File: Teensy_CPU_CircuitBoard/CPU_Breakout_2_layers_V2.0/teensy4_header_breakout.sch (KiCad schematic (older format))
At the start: 0 parts

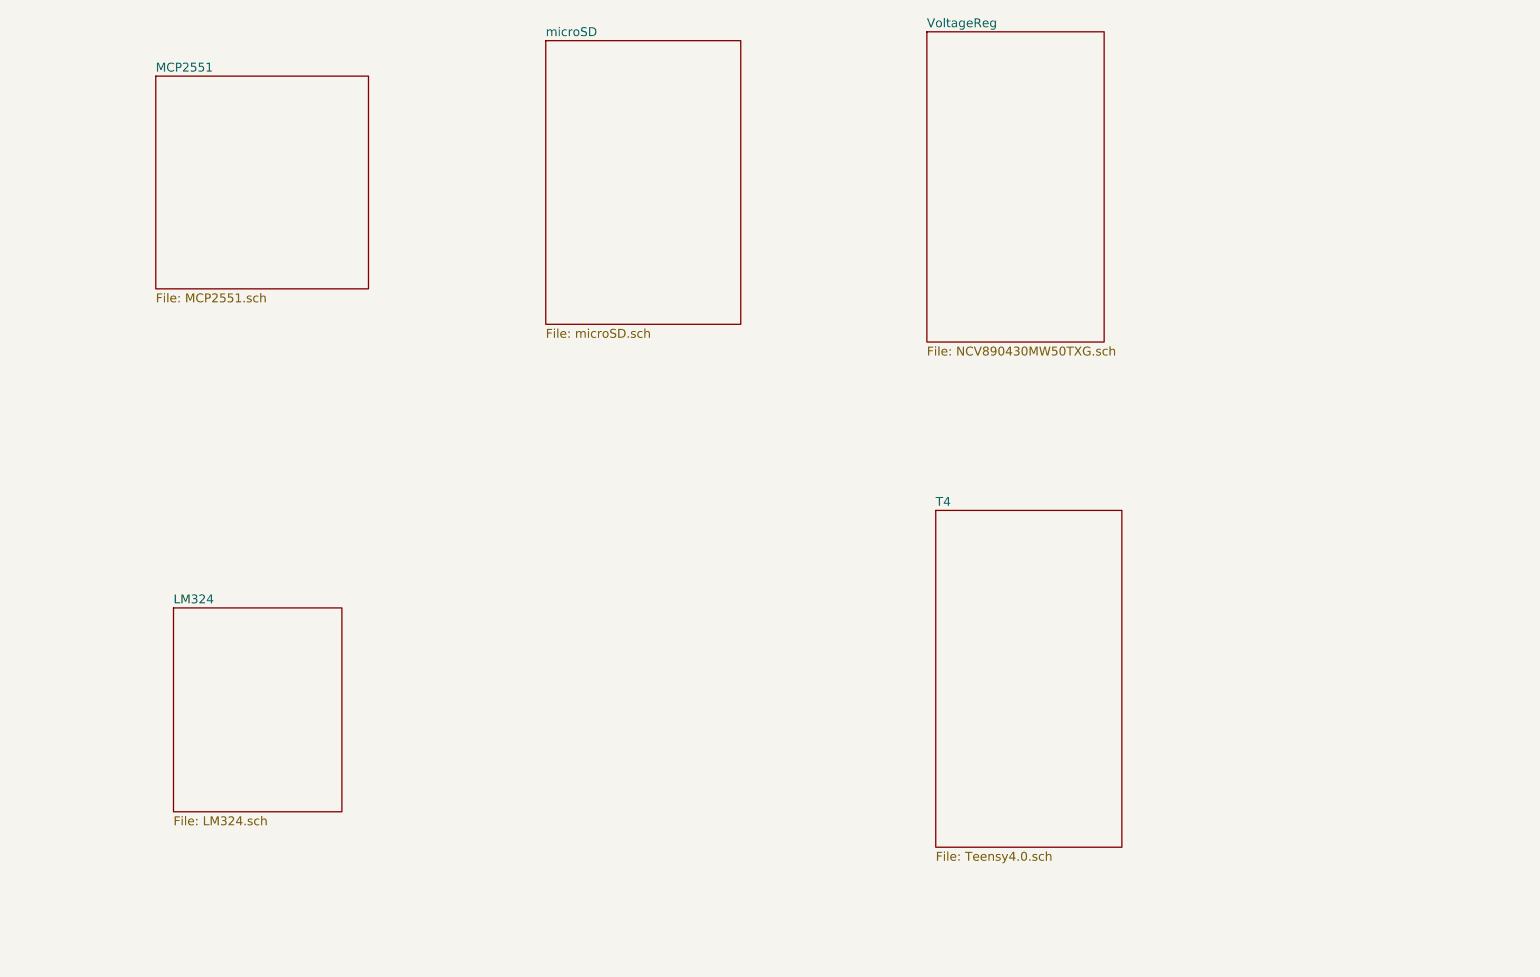
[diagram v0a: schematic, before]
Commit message: Start of V3 STM32
Imported symbols/footprints ...
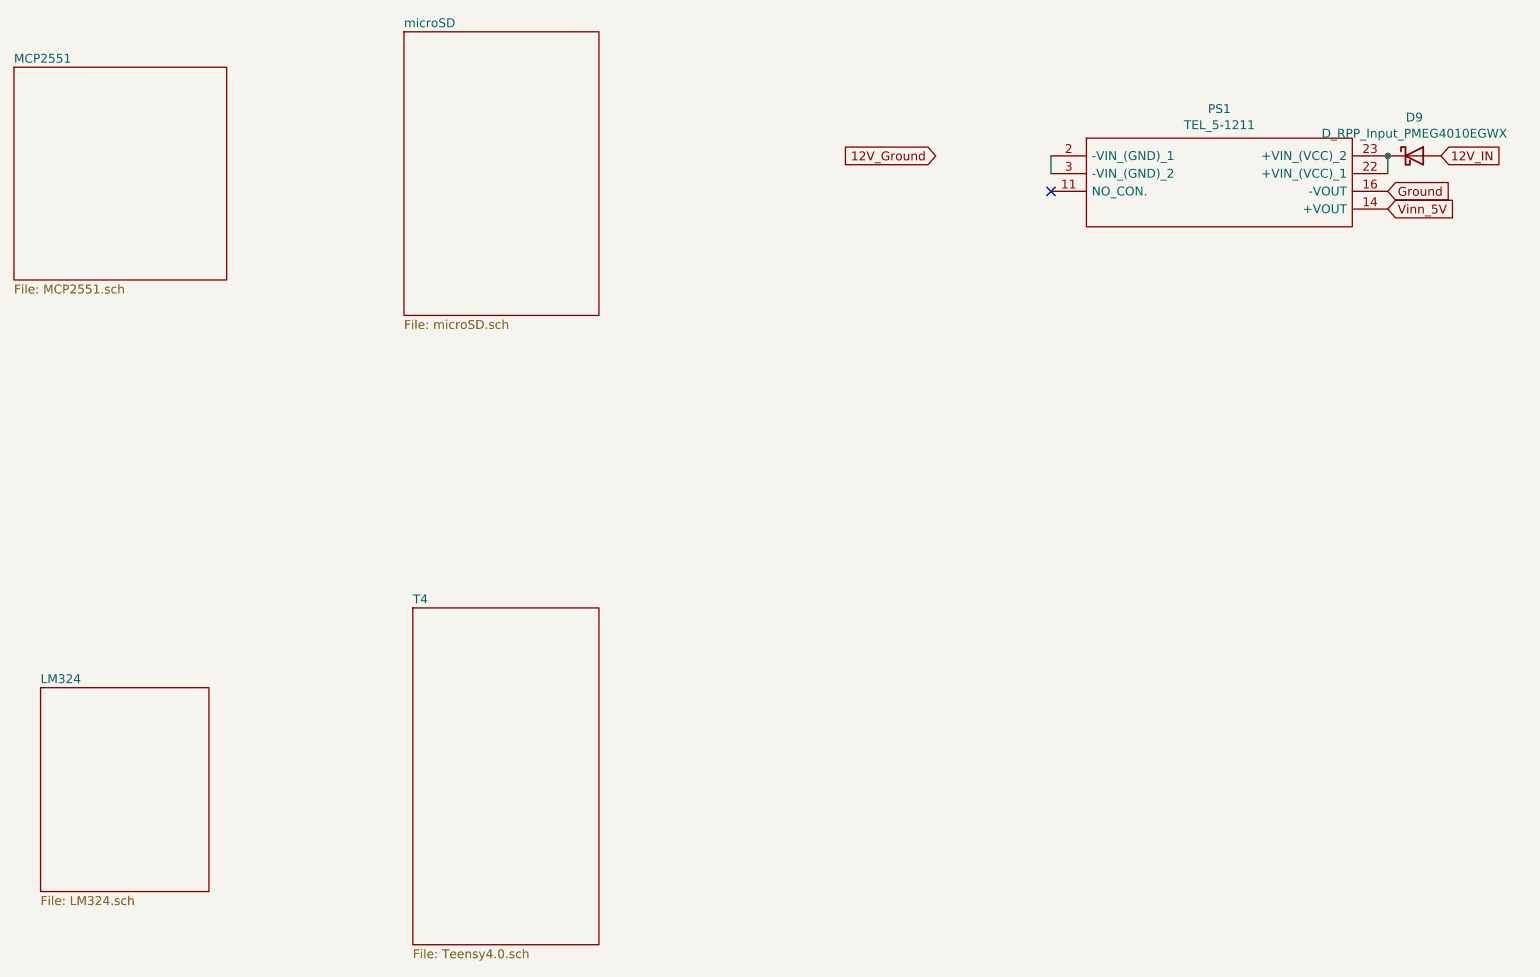
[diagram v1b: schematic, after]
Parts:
- added D9: D_RPP_Input_PMEG4010EGWX, Teensy_Footprint_Library:D_RPP_PMEG4010EGWX, symbol teensy4_header_breakout-cache:D_RPP_Input_PMEG4010EGWX
- added PS1: TEL_5-1211, Teensy_Footprint_Library:TEL51211, symbol teensy4_header_breakout-cache:TEL_5-1211
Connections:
- new net: PS1.2 (-VIN_(GND)_1), PS1.3 (-VIN_(GND)_2)
- new net: D9.1 (K), PS1.22 (+VIN_(VCC)_1), PS1.23 (+VIN_(VCC)_2)
- new net 12V_IN: D9.2 (A)
- new net Ground: PS1.16 (-VOUT)
- new net Vinn_5V: PS1.14 (+VOUT)
- no-connect marks 0 -> 1
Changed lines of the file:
@@
 $Descr A4 11693 8268
 encoding utf-8
-Sheet 1 6
+Sheet 1 5
 Title ""
 Date ""
@@
 $EndDescr
 $Sheet
-S 2400 4200 950  1150
+S 1650 4650 950  1150
 U 5DE81E30
 F0 "LM324" 50
@@
 $EndSheet
 $Sheet
-S 2300 1200 1200 1200
+S 1500 1150 1200 1200
 U 5DE8C472
 F0 "MCP2551" 50
@@
 $EndSheet
 $Sheet
-S 4500 1000 1100 1600
+S 3700 950  1100 1600
 U 5DE8C4DF
 F0 "microSD" 50
@@
 $EndSheet
 $Sheet
-S 6650 950  1000 1750
-U 5DE8C550
-F0 "VoltageReg" 50
-F1 "NCV890430MW50TXG.sch" 50
-$EndSheet
-$Sheet
-S 6700 3650 1050 1900
+S 3750 4200 1050 1900
 U 5DE8C5CE
 F0 "T4" 50
 F1 "Teensy4.0.sch" 50
 $EndSheet
+Text GLabel 9550 1650 2    50   Input ~ 0
+12V_IN
+Text GLabel 9250 1950 2    50   Input ~ 0
+Vinn_5V
+Text GLabel 6700 1650 0    50   Input ~ 0
+12V_Ground
+$Comp
+L teensy4_header_breakout-cache:TEL_5-1211 PS1
+U 1 1 5FAC174D
+P 7350 1650
+F 0 "PS1" H 8300 1915 50  0000 C CNN
+F 1 "TEL_5-1211" H 8300 1824 50  0000 C CNN
+F 2 "Teensy_Footprint_Library:TEL51211" H 9100 1750 50  0001 L CNN
+F 3 "https://www.tracopower.com/products/tel5.pdf" H 9100 1650 50  0001 L CNN
+F 4 "TEL5 DC-DC converter,9-18Vin 5V 5W TRACOPOWER Isolated DC-DC Converter, Vin 9  18 V dc, Vout 5V dc, I/O isolation 1500V dc" H 9100 1550 50  0001 L CNN "Description"
+F 5 "10.45" H 9100 1450 50  0001 L CNN "Height"
+F 6 "Traco Power" H 9100 1350 50  0001 L CNN "Manufacturer_Name"
+F 7 "TEL 5-1211" H 9100 1250 50  0001 L CNN "Manufacturer_Part_Number"
+F 8 "495-TEL-5-1211" H 9100 950 50  0001 L CNN "Mouser Part Number"
+F 9 "https://www.mouser.co.uk/ProductDetail/TRACO-Power/TEL-5-1211?qs=ckJk83FOD0WBOuRLitdGqQ%3D%3D" H 9100 850 50  0001 L CNN "Mouser Price/Stock"
+	1    7350 1650
+	1    0    0    -1
+$EndComp
+NoConn ~ 7350 1850
+Text GLabel 9250 1850 2    50   Input ~ 0
+Ground
+Wire Wire Line
+	9250 1750 9250 1650
+Wire Wire Line
+	7350 1650 7350 1750
+$Comp
+L teensy4_header_breakout-cache:D_RPP_Input_PMEG4010EGWX D9
+U 1 1 5FACD4C4
+P 9400 1650
+F 0 "D9" H 9400 1867 50  0000 C CNN
+F 1 "D_RPP_Input_PMEG4010EGWX" H 9400 1776 50  0000 C CNN
+F 2 "Teensy_Footprint_Library:D_RPP_PMEG4010EGWX" H 9400 1650 50  0001 C CNN
+F 3 "~" H 9400 1650 50  0001 C CNN
+	1    9400 1650
+	1    0    0    -1
+$EndComp
+Connection ~ 9250 1650
 $EndSCHEMATC
